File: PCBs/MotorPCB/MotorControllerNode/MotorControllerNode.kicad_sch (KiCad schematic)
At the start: 30 parts, among them IC1 DAC53202RTER, IC2 TXS0108EQPWRQ1, IC3 TXS0108EQPWRQ1, J2 DSUB9 J1, J3 Encoder, J4 GPIO, J5 DSUB9 to backplane, J6 Battery negative, J7 Reversing contactor 1, J8 Reversing contactor 2, J9 DSUB15 J2, Q1 NPN, U1 ESP32-S3-DevKitC, U2 SN65HVD230, U3 J104D2C5VDC.20S

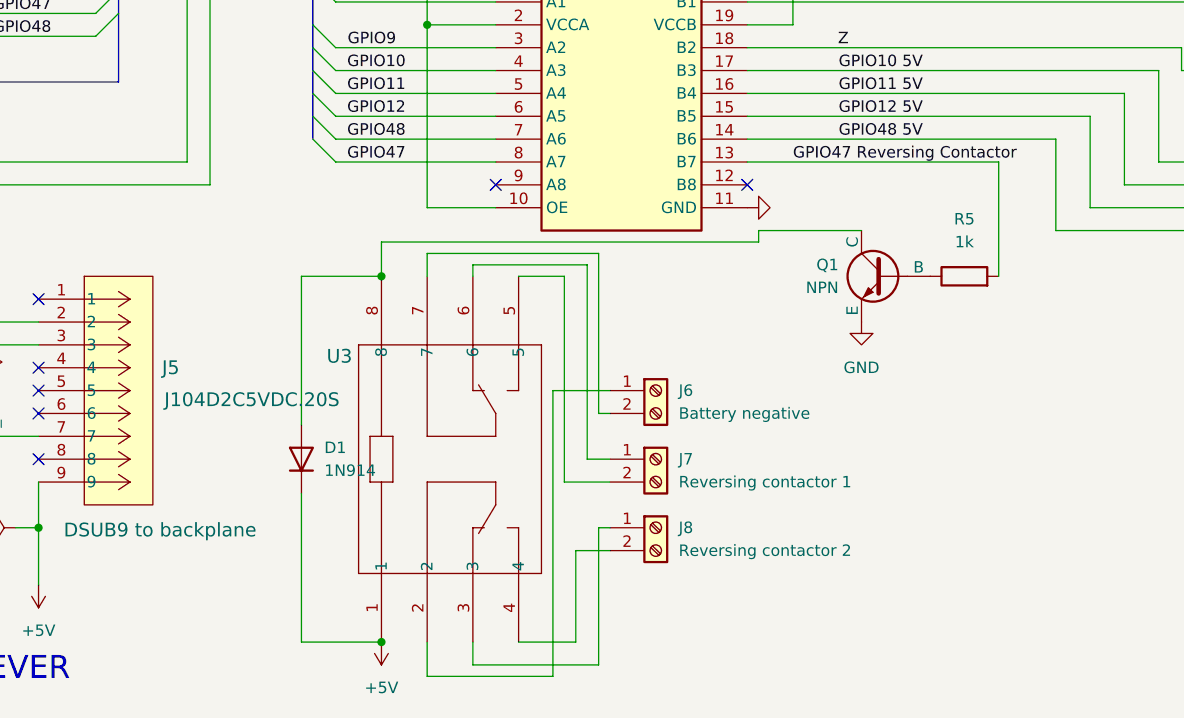
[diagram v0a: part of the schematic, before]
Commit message: Revert "added driver controls v2"
This reverts commit c73e8f860f70517a898f0b3e351800c05ab551df.
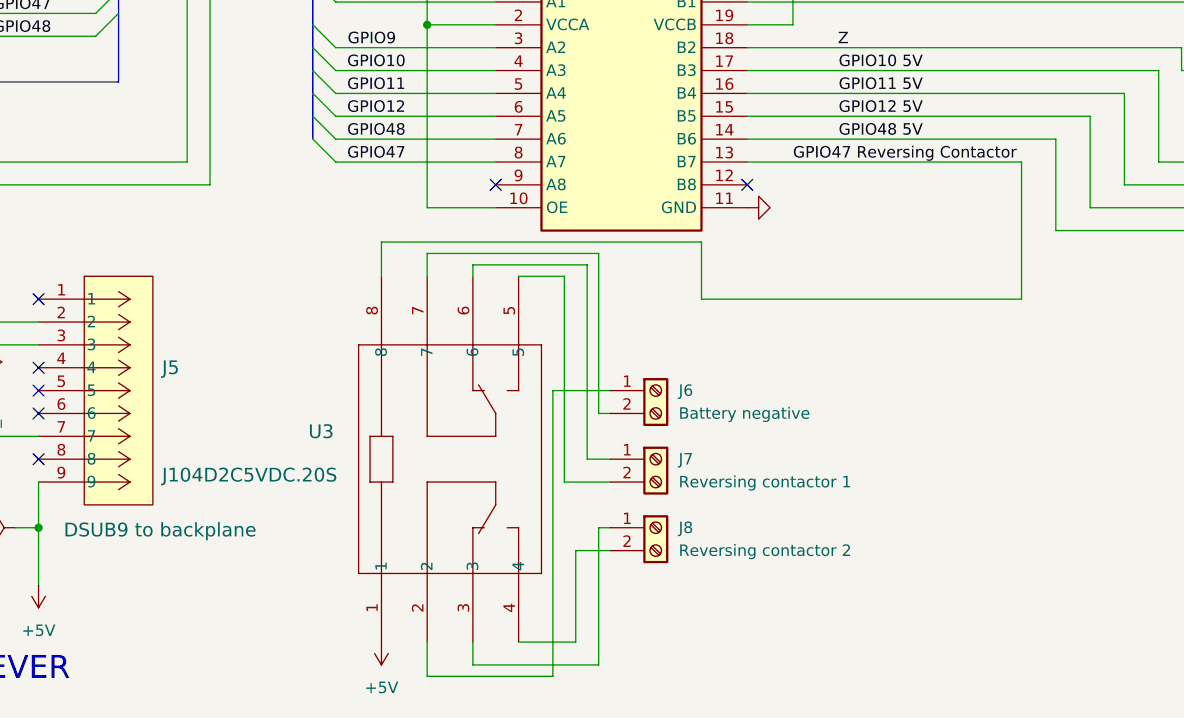
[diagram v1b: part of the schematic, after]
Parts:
- removed D1: 1N914, Diode_THT:D_DO-35_SOD27_P7.62mm_Horizontal, symbol Diode:1N914
- removed Q1: NPN, Package_TO_SOT_THT:TO-92, symbol Simulation_SPICE:NPN
- removed R5: 1k, Resistor_SMD:R_0603_1608Metric_Pad0.98x0.95mm_HandSolder, symbol Device:R
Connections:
- net GPIO47 Reversing Contactor: now also U3.8

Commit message: Reapply "added driver controls v2"
This reverts commit d70487c3c1110107dce6cdfc2b36a156bfb5c696.
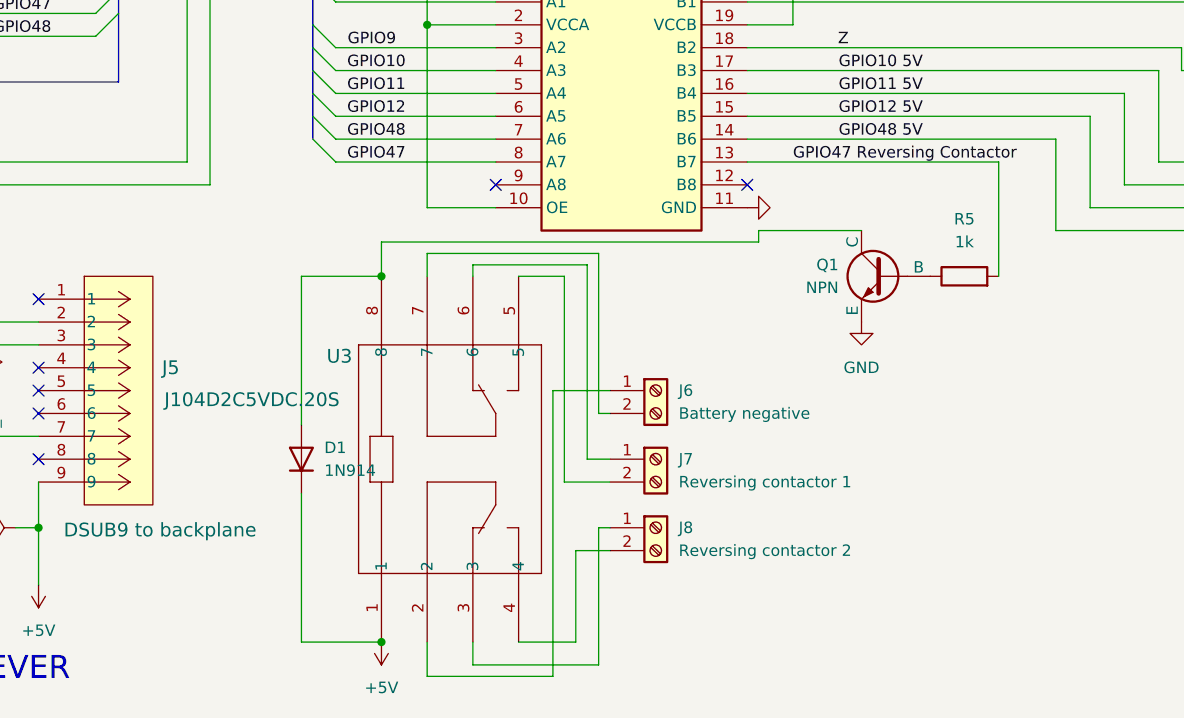
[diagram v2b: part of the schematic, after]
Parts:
- added D1: 1N914, Diode_THT:D_DO-35_SOD27_P7.62mm_Horizontal, symbol Diode:1N914
- added Q1: NPN, Package_TO_SOT_THT:TO-92, symbol Simulation_SPICE:NPN
- added R5: 1k, Resistor_SMD:R_0603_1608Metric_Pad0.98x0.95mm_HandSolder, symbol Device:R
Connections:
- net +5V: now also D1.1 (K)
- net GND: now also Q1.1 (E)
- net GPIO47 Reversing Contactor: now also R5.2; no longer U3.8
- new net: D1.2 (A), Q1.3 (C), U3.8
- new net: Q1.2 (B), R5.1
